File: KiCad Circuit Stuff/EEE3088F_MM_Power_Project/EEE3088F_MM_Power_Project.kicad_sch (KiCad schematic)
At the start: 60 parts, among them J1 Conn_02x16_Odd_Even, J2 Conn_01x02, U1 MT3608, U2 AMS1117-3.3, U3 TP4056, U4 INA219AIDCNR, U6 TS5A3159DCKR, U7 TPS5430DDAR

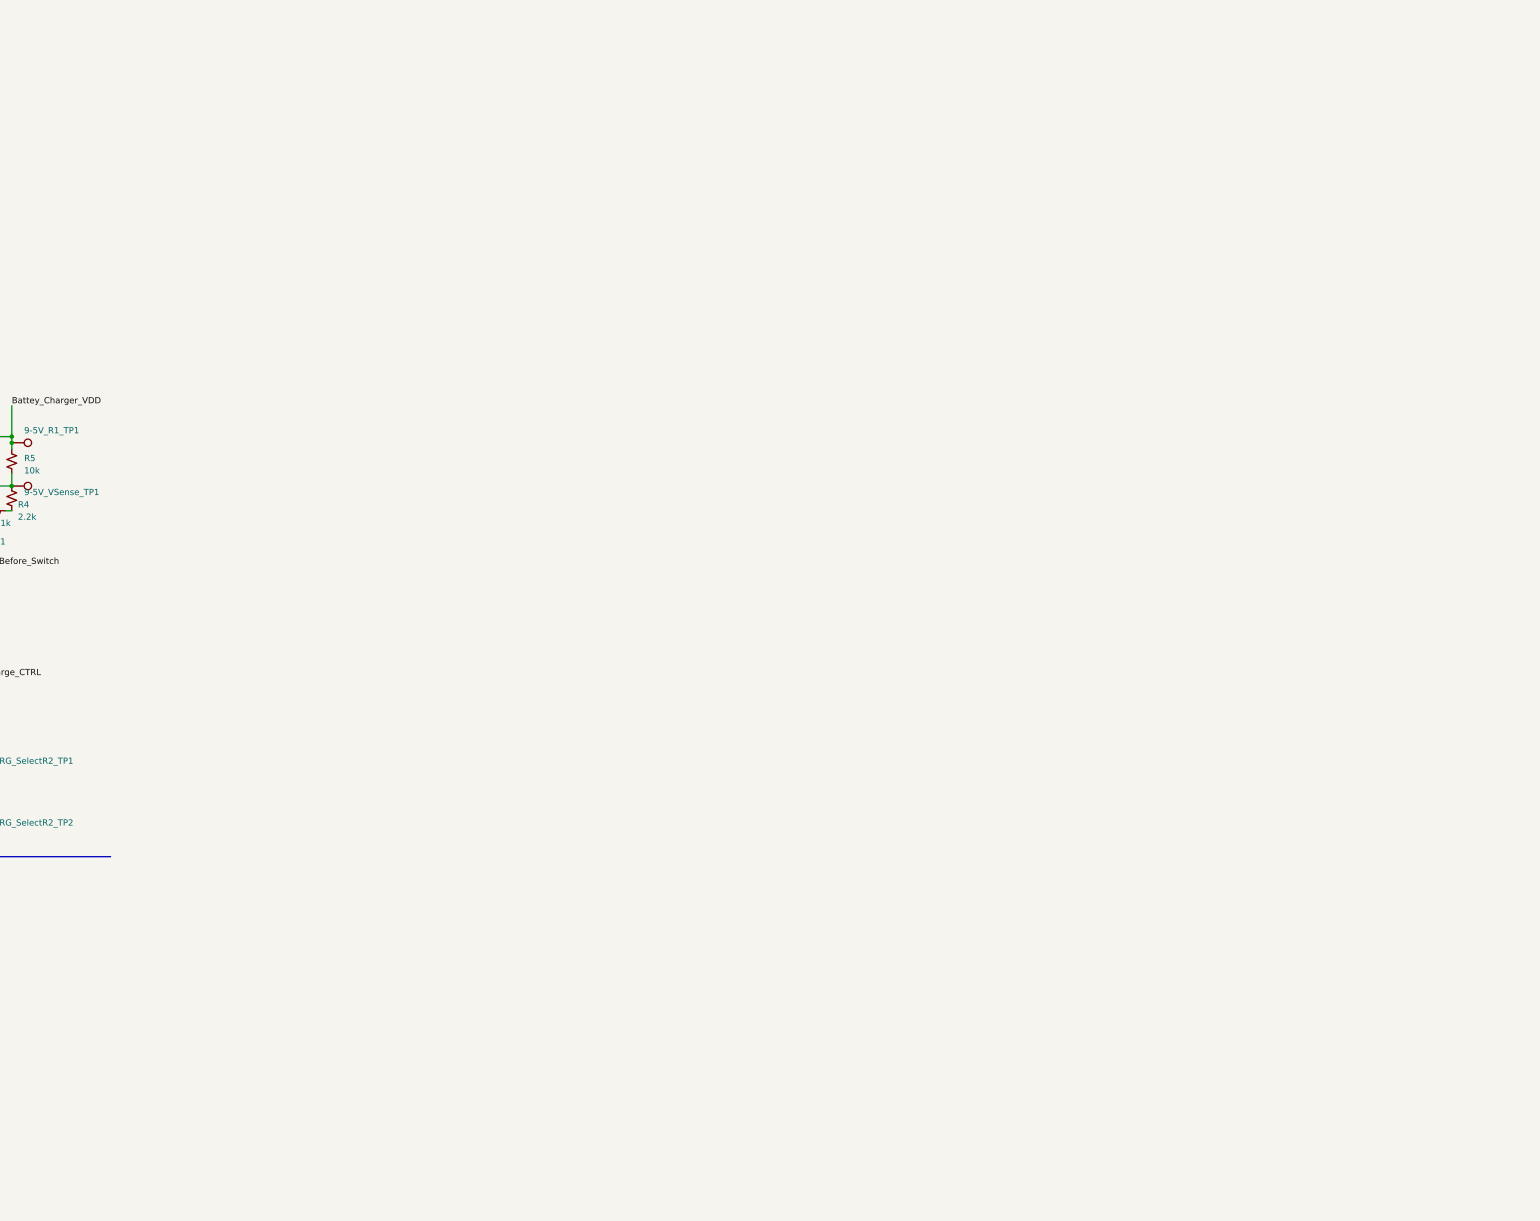
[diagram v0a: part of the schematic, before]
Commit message: added some stuff
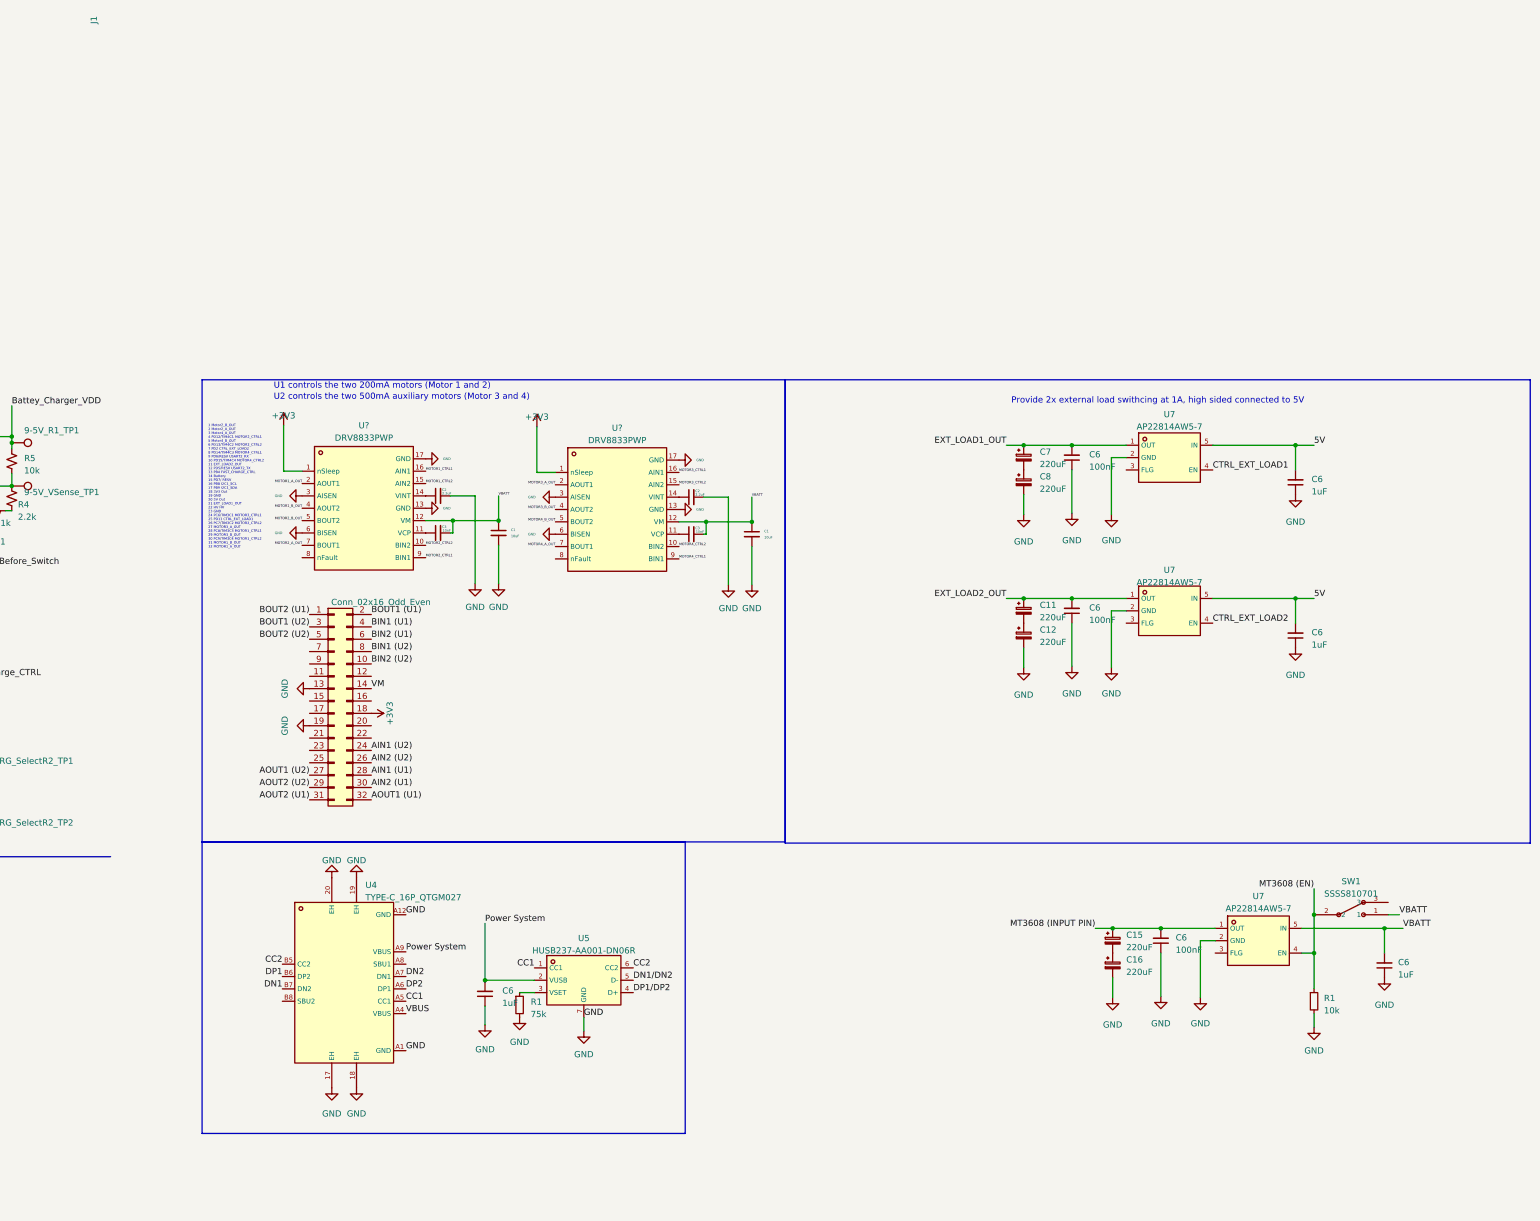
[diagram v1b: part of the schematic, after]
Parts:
- added C1 (x2): 10uF, Capacitor_SMD:C_0603_1608Metric_Pad1.08x0.95mm_HandSolder, symbol Device:C_Small
- added C11, C12, C15, C16, C7, C8: 220uF, Capacitor_SMD:C_Elec_6.3x7.7, symbol Device:C_Polarized_Small
- added C2 (x2): 2.2uF, Capacitor_SMD:C_0402_1005Metric_Pad0.74x0.62mm_HandSolder, symbol Device:C_Small
- added C3 (x2): 10nF, Capacitor_SMD:C_0402_1005Metric_Pad0.74x0.62mm_HandSolder, symbol Device:C_Small
- added C6 (x3): 100nF, Capacitor_SMD:C_0402_1005Metric_Pad0.74x0.62mm_HandSolder, symbol Device:C_Small
- added C6 (x4): 1uF, Capacitor_SMD:C_0402_1005Metric_Pad0.74x0.62mm_HandSolder, symbol Device:C_Small
- added J1: Conn_02x16_Odd_Even, symbol Connector_Generic:Conn_02x16_Odd_Even
- added R1: 75k, Resistor_SMD:R_0603_1608Metric_Pad0.98x0.95mm_HandSolder, symbol Device:R_Small
- added R1: 10k, Resistor_SMD:R_0603_1608Metric_Pad0.98x0.95mm_HandSolder, symbol Device:R_Small
- added SW1: SSSS810701, footprint:SW-SMD_SSSS810701, symbol SSSS810701:SSSS810701
- added U4: TYPE-C_16P_QTGM027, DRV8833_NEW:USB-C-SMD_TYPE-C-16P-QTGM027, symbol TYPE-C 16P QTGM027:TYPE-C_16P_QTGM027
- added U5: HUSB237-AA001-DN06R, DRV8833_NEW:TDFN-6_L2.0-W2.0-P0.65-TL-EP, symbol HUSB237_NEW:HUSB237-AA001-DN06R
- added U7 (x3): AP22814AW5-7, DRV8833_NEW:SOT-25_L3.0-W1.6-P0.95-LS2.8-BL, symbol AP22814AW5-7:AP22814AW5-7
- added U? (x2): DRV8833PWP, DRV8833_NEW:TSSOP-16_L5.0-W4.4-P0.65-LS6.4-BL-EP, symbol DRV8833_NEW:DRV8833PWP
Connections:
- net +3V3: now also J1.18 (Pin_18), U?.1 (nSleep), U?.1 (nSleep)
- net GND: now also C1.2, C1.2, C12.2, C16.2, C2.2, C2.2, C6.1, C6.1, C6.1, C6.1, C6.1, C6.1, C6.1, C8.2, J1.13 (Pin_13), J1.19 (Pin_19), R1.2, R1.2, U4.17 (EH), U4.18 (EH), U4.19 (EH), U4.20 (EH), U4.A1 (GND), U4.A12 (GND), U5.7 (GND), U7.2 (GND), U7.2 (GND), U7.2 (GND), U?.13 (GND), U?.13 (GND), U?.17 (GND), U?.17 (GND), U?.3 (AISEN), U?.3 (AISEN), U?.6 (BISEN), U?.6 (BISEN)
- new net: C15.2, C16.1
- new net: C7.2, C8.1
- new net: C2.1, U?.14 (VINT) (x2)
- new net: C3.1, U?.11 (VCP) (x2)
- new net: R1.1, U5.3 (VSET)
- new net: C11.2, C12.1
- new net 5V: C6.2, C6.2, U7.5 (IN), U7.5 (IN)
- new net AIN1 (U1): J1.28 (Pin_28)
- new net AIN1 (U2): J1.24 (Pin_24)
- new net AIN2 (U1): J1.30 (Pin_30)
- new net AIN2 (U2): J1.26 (Pin_26)
- new net AOUT1 (U1): J1.32 (Pin_32)
- new net AOUT1 (U2): J1.27 (Pin_27)
- new net AOUT2 (U1): J1.31 (Pin_31)
- new net AOUT2 (U2): J1.29 (Pin_29)
- new net BIN1 (U1): J1.4 (Pin_4)
- new net BIN1 (U2): J1.8 (Pin_8)
- new net BIN2 (U1): J1.6 (Pin_6)
- new net BIN2 (U2): J1.10 (Pin_10)
- new net BOUT1 (U1): J1.2 (Pin_2)
- new net BOUT1 (U2): J1.3 (Pin_3)
- new net BOUT2 (U1): J1.1 (Pin_1)
- new net BOUT2 (U2): J1.5 (Pin_5)
- new net CC1: U4.A5 (CC1), U5.1 (CC1)
- new net CC2: U4.B5 (CC2), U5.6 (CC2)
- new net CTRL_EXT_LOAD1: U7.4 (EN)
- new net CTRL_EXT_LOAD2: U7.4 (EN)
- new net DN1: U4.B7 (DN2)
- new net DN1/DN2: U5.5 (D-)
- new net DN2: U4.A7 (DN1)
- new net DP1: U4.B6 (DP2)
- new net DP1/DP2: U5.4 (D+)
- new net DP2: U4.A6 (DP1)
- new net EXT_LOAD1_OUT: C6.2, C7.1, U7.1 (OUT)
- new net EXT_LOAD2_OUT: C11.1, C6.2, U7.1 (OUT)
- new net MOTOR1_A_OUT: U?.2 (AOUT1)
- new net MOTOR1_B_OUT: U?.4 (AOUT2)
- new net MOTOR1_CTRL1: U?.16 (AIN1)
- new net MOTOR1_CTRL2: U?.15 (AIN2)
- new net MOTOR2_A_OUT: U?.7 (BOUT1)
- new net MOTOR2_B_OUT: U?.5 (BOUT2)
- new net MOTOR2_CTRL1: U?.9 (BIN1)
- new net MOTOR2_CTRL2: U?.10 (BIN2)
- new net MOTOR3_A_OUT: U?.2 (AOUT1)
- new net MOTOR3_B_OUT: U?.4 (AOUT2)
- new net MOTOR3_CTRL1: U?.16 (AIN1)
- new net MOTOR3_CTRL2: U?.15 (AIN2)
- new net MOTOR4_A_OUT: U?.7 (BOUT1)
- new net MOTOR4_B_OUT: U?.5 (BOUT2)
- new net MOTOR4_CTRL1: U?.9 (BIN1)
- new net MOTOR4_CTRL2: U?.10 (BIN2)
- new net MT3608 (EN): R1.1, SW1.2, U7.4 (EN)
- new net MT3608 (INPUT PIN): C15.1, C6.2, U7.1 (OUT)
- new net Power System: C6.2, U4.A9 (VBUS), U5.2 (VUSB)
- new net VBATT: C1.1, C1.1, C3.2, C3.2, C6.2, SW1.1, U7.5 (IN), U?.12 (VM), U?.12 (VM)
- new net VBUS: U4.A4 (VBUS)
- new net VM: J1.14 (Pin_14)
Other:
- note added: "1 Motor2_B_OUT 2 Motor2_A_OUT 3 Motor4_A_OUT 4 PD12/TIM4C1 MOTOR2_CTRL1 5 Motor4_B_OUT 6 PD13/TIM4C2 MOTOR2_CTRL2 7 PD2 CTRL_EXT_LOAD2 8 PD14/TIM4C3 MOTOR4_CTRL1 9 PD6/RESV USART2_RX 10 PD15/TIM4C4 MOTOR4_CTRL2 11 EXT_LOAD2_OUT 12 PD5/RESV USART2_TX 13 PB4 FAST_CHARGE_CTRL 14 Battery 15 PD7/ RESV 16 PB8 I2C1_SCL 17 PB9 I2C1_SDA 18 3V3 Out 19 GND 20 5V Out 21 EXT_LOAD1_OUT 22 HV HV 23 GND 24 PC6/T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"
- note added: "Provide 2x external load swithcing at 1A, high sided connected to 5V"
- note added: "U1 controls the two 200mA motors (Motor 1 and 2)"
- note added: "U2 controls the two 500mA auxiliary motors (Motor 3 and 4)"
